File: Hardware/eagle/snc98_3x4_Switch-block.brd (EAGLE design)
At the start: 57.5 x 84.2 mm, 67 parts

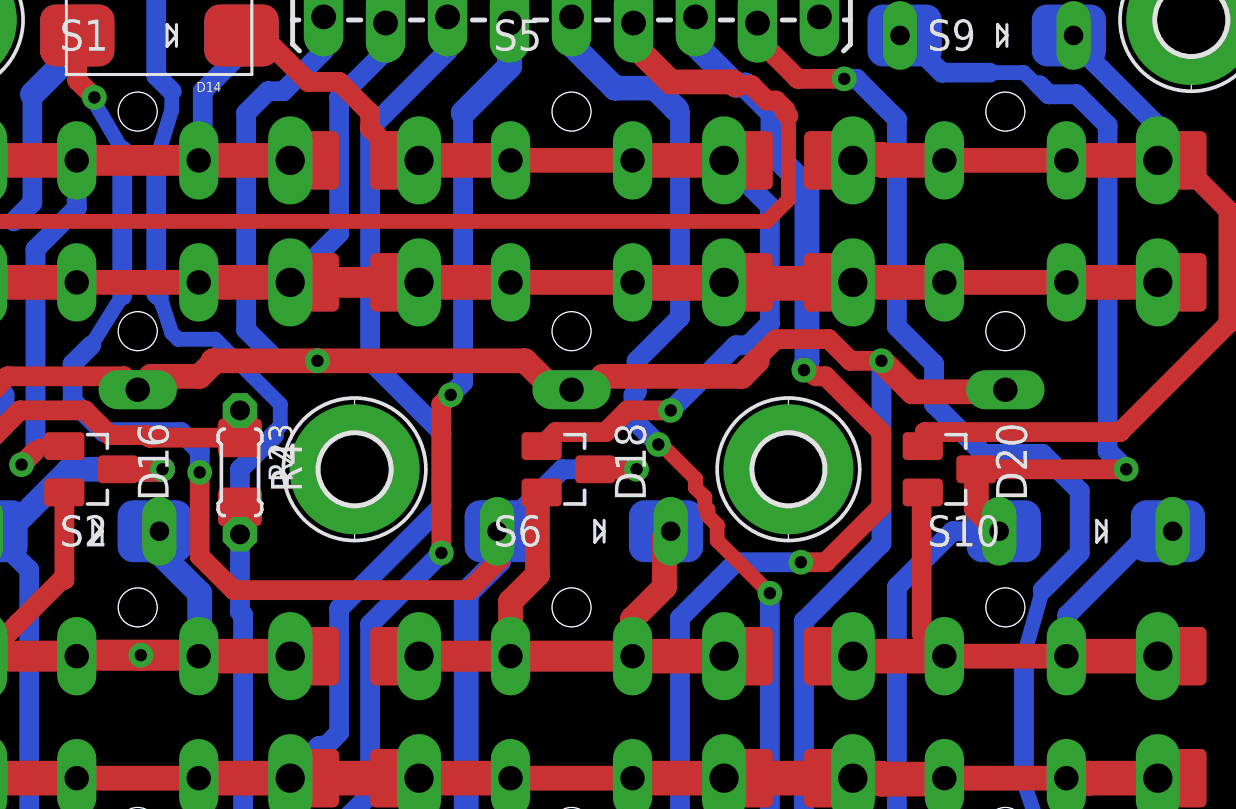
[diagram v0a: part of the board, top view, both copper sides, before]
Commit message: New Picture "Switch mechanical"
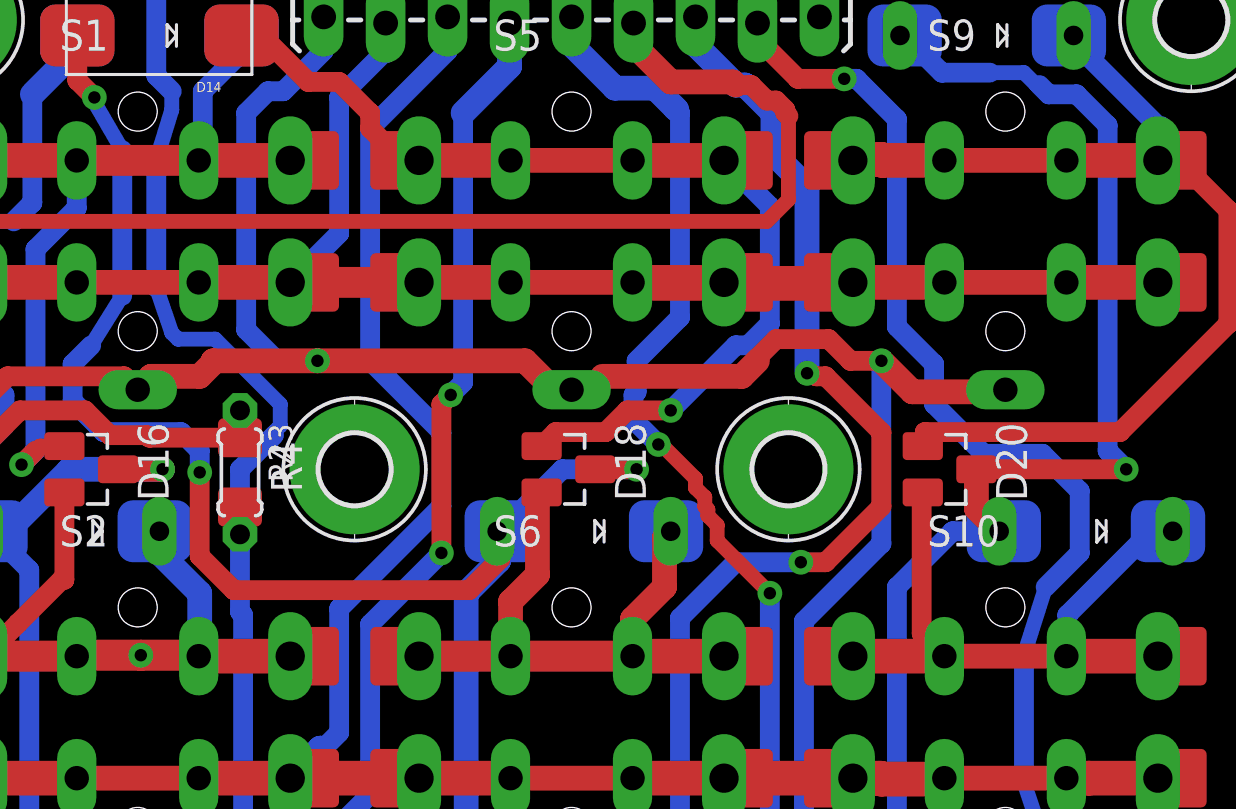
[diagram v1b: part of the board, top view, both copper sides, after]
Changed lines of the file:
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@@
 <setting verticaltext="up"/>
 </settings>
-<grid distance="5" unitdist="mil" unit="mil" style="dots" multiple="1" display="yes" altdistance="0.005" altunitdist="inch" altunit="inch"/>
+<grid distance="5" unitdist="mil" unit="mm" style="dots" multiple="1" display="yes" altdistance="0.005" altunitdist="inch" altunit="inch"/>
 <layers>
 <layer number="1" name="Top" color="4" fill="1" visible="yes" active="yes"/>
@@
 <layer number="21" name="tPlace" color="16" fill="1" visible="yes" active="yes"/>
 <layer number="22" name="bPlace" color="14" fill="1" visible="yes" active="yes"/>
-<layer number="23" name="tOrigins" color="15" fill="1" visible="no" active="yes"/>
-<layer number="24" name="bOrigins" color="15" fill="1" visible="no" active="yes"/>
-<layer number="25" name="tNames" color="7" fill="1" visible="yes" active="yes"/>
-<layer number="26" name="bNames" color="7" fill="1" visible="yes" active="yes"/>
+<layer number="23" name="tOrigins" color="15" fill="1" visible="yes" active="yes"/>
+<layer number="24" name="bOrigins" color="15" fill="1" visible="yes" active="yes"/>
+<layer number="25" name="tNames" color="7" fill="1" visible="no" active="yes"/>
+<layer number="26" name="bNames" color="7" fill="1" visible="no" active="yes"/>
 <layer number="27" name="tValues" color="7" fill="1" visible="no" active="yes"/>
 <layer number="28" name="bValues" color="7" fill="1" visible="no" active="yes"/>
@@
 <layer number="45" name="Holes" color="7" fill="1" visible="yes" active="yes"/>
 <layer number="46" name="Milling" color="3" fill="1" visible="no" active="yes"/>
-<layer number="47" name="Measures" color="7" fill="1" visible="no" active="yes"/>
-<layer number="48" name="Document" color="7" fill="1" visible="yes" active="yes"/>
+<layer number="47" name="Measures" color="7" fill="1" visible="yes" active="yes"/>
+<layer number="48" name="Document" color="7" fill="1" visible="no" active="yes"/>
 <layer number="49" name="Reference" color="7" fill="1" visible="no" active="yes"/>
 <layer number="50" name="dxf" color="7" fill="1" visible="no" active="yes"/>
@@
 <text x="2.667" y="23.622" size="1.27" layer="22" ratio="16" rot="MR270" align="center">source</text>
 <text x="28.448" y="1.905" size="1.27" layer="22" ratio="16" rot="MR0" align="center">https://oshpark.com/profiles/Jens_G</text>
-<dimension x1="0" y1="-3.81" x2="57.15" y2="-3.81" x3="28.575" y3="-3.81" textsize="1.778" textratio="15" layer="47" dtype="radius"/>
-<dimension x1="-3.81" y1="0" x2="-3.81" y2="83.82" x3="-3.81" y3="41.91" textsize="1.778" textratio="15" layer="47" dtype="radius"/>
 <wire x1="0" y1="84.201" x2="57.531" y2="84.201" width="0" layer="20"/>
 <wire x1="57.531" y1="84.201" x2="57.531" y2="0" width="0" layer="20"/>
@@
 <wire x1="46.5455" y1="80.5815" x2="46.5455" y2="80.137" width="0.127" layer="21"/>
 <wire x1="46.5455" y1="80.137" x2="46.5455" y2="79.6925" width="0.127" layer="21"/>
+<dimension x1="10.922" y1="31.877" x2="10.922" y2="52.197" x3="-1.905" y3="42.037" textsize="1.778" textratio="15" layer="47"/>
+<dimension x1="0" y1="0" x2="0" y2="84.201" x3="-6.477" y3="42.1005" textsize="1.778" textratio="15" layer="47"/>
+<dimension x1="0" y1="0" x2="57.531" y2="0" x3="28.7655" y3="-10.668" textsize="1.778" textratio="15" layer="47"/>
+<dimension x1="10.922" y1="11.557" x2="28.702" y2="11.557" x3="19.812" y3="-4.445" textsize="1.778" textratio="15" layer="47"/>
 </plain>
 <attributes>
@@
 <wire x1="48.006" y1="62.992" x2="49.53" y2="61.468" width="0.8128" layer="16"/>
 <wire x1="49.53" y1="61.468" x2="49.53" y2="58.928" width="0.8128" layer="16"/>
-<wire x1="49.53" y1="58.928" x2="48.006" y2="57.404" width="0.8128" layer="16"/>
-<wire x1="48.006" y1="57.404" x2="47.244" y2="54.737" width="0.6096" layer="16"/>
+<wire x1="49.53" y1="58.928" x2="48.133" y2="57.531" width="0.8128" layer="16"/>
+<wire x1="48.133" y1="57.531" x2="47.244" y2="54.737" width="0.6096" layer="16"/>
 <wire x1="47.244" y1="54.737" x2="47.244" y2="49.53" width="0.8128" layer="16"/>
 <wire x1="47.244" y1="49.53" x2="48.006" y2="47.244" width="0.6096" layer="16"/>
@@
 <wire x1="36.957" y1="76.962" x2="36.957" y2="75.311" width="1.016" layer="16"/>
 <wire x1="36.957" y1="75.311" x2="38.354" y2="73.914" width="1.016" layer="16"/>
-<wire x1="38.354" y1="73.914" x2="38.354" y2="66.802" width="1.016" layer="16"/>
-<wire x1="38.354" y1="66.802" x2="38.227" y2="66.421" width="1.016" layer="16"/>
-<via x="38.227" y="66.421" extent="1-16" drill="0.508"/>
-<wire x1="38.227" y1="66.421" x2="38.735" y2="66.167" width="0.8128" layer="1"/>
+<wire x1="38.354" y1="73.914" x2="38.354" y2="66.294" width="1.016" layer="16"/>
+<via x="38.354" y="66.294" extent="1-16" drill="0.508"/>
+<wire x1="38.354" y1="66.294" x2="38.735" y2="66.167" width="0.8128" layer="1"/>
 <wire x1="38.735" y1="66.167" x2="39.116" y2="66.167" width="0.8128" layer="1"/>
 <wire x1="39.116" y1="66.167" x2="41.402" y2="63.881" width="0.8128" layer="1"/>
@@
 <wire x1="14.097" y1="67.691" x2="12.573" y2="67.691" width="0.6096" layer="16"/>
 <wire x1="12.573" y1="67.691" x2="12.319" y2="67.945" width="0.6096" layer="16"/>
-<wire x1="12.319" y1="67.945" x2="11.938" y2="69.088" width="0.6096" layer="16"/>
 <wire x1="11.684" y1="82.423" x2="12.192" y2="82.931" width="0.8128" layer="16"/>
 <via x="12.192" y="82.931" extent="1-16" drill="0.508"/>
@@
 <wire x1="38.989" y1="81.915" x2="38.989" y2="81.026" width="0.8128" layer="1"/>
 <wire x1="38.989" y1="81.026" x2="38.862" y2="80.899" width="0.8128" layer="1"/>
-<wire x1="11.684" y1="69.85" x2="11.684" y2="69.723" width="0.6096" layer="16"/>
-<wire x1="11.684" y1="69.723" x2="11.7978625" y2="69.43834375" width="0.6096" layer="16"/>
-<wire x1="11.7978625" y1="69.43834375" x2="11.938" y2="69.088" width="0.6096" layer="16"/>
+<wire x1="11.684" y1="69.85" x2="11.684" y2="69.80620625" width="0.6096" layer="16"/>
 <wire x1="37.719" y1="83.185" x2="38.989" y2="81.915" width="0.8128" layer="1"/>
 <wire x1="37.719" y1="83.185" x2="34.417" y2="83.185" width="0.8128" layer="1"/>
@@
 <wire x1="11.811" y1="75.438" x2="11.811" y2="75.311" width="0.6096" layer="16"/>
 <wire x1="11.811" y1="75.311" x2="11.684" y2="75.184" width="0.6096" layer="16"/>
-<wire x1="11.684" y1="75.184" x2="11.684" y2="69.55220625" width="0.8128" layer="16"/>
-<wire x1="11.684" y1="69.55220625" x2="11.7978625" y2="69.43834375" width="0.8128" layer="16"/>
+<wire x1="11.684" y1="75.184" x2="11.684" y2="69.80620625" width="0.8128" layer="16"/>
 <wire x1="55.499" y1="20.955" x2="55.499" y2="22.479" width="0.8128" layer="1"/>
 <wire x1="55.499" y1="23.597" x2="55.499" y2="22.479" width="0.8128" layer="1"/>
@@
 <via x="16.002" y="43.434" extent="1-16" drill="0.508"/>
 <wire x1="16.002" y1="43.434" x2="31.75" y2="43.434" width="0.8128" layer="1"/>
+<wire x1="12.319" y1="67.945" x2="11.684" y2="69.80620625" width="0.6096" layer="16"/>
 </signal>
 <signal name="A_1">
